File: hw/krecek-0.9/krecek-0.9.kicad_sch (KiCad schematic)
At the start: 0 parts

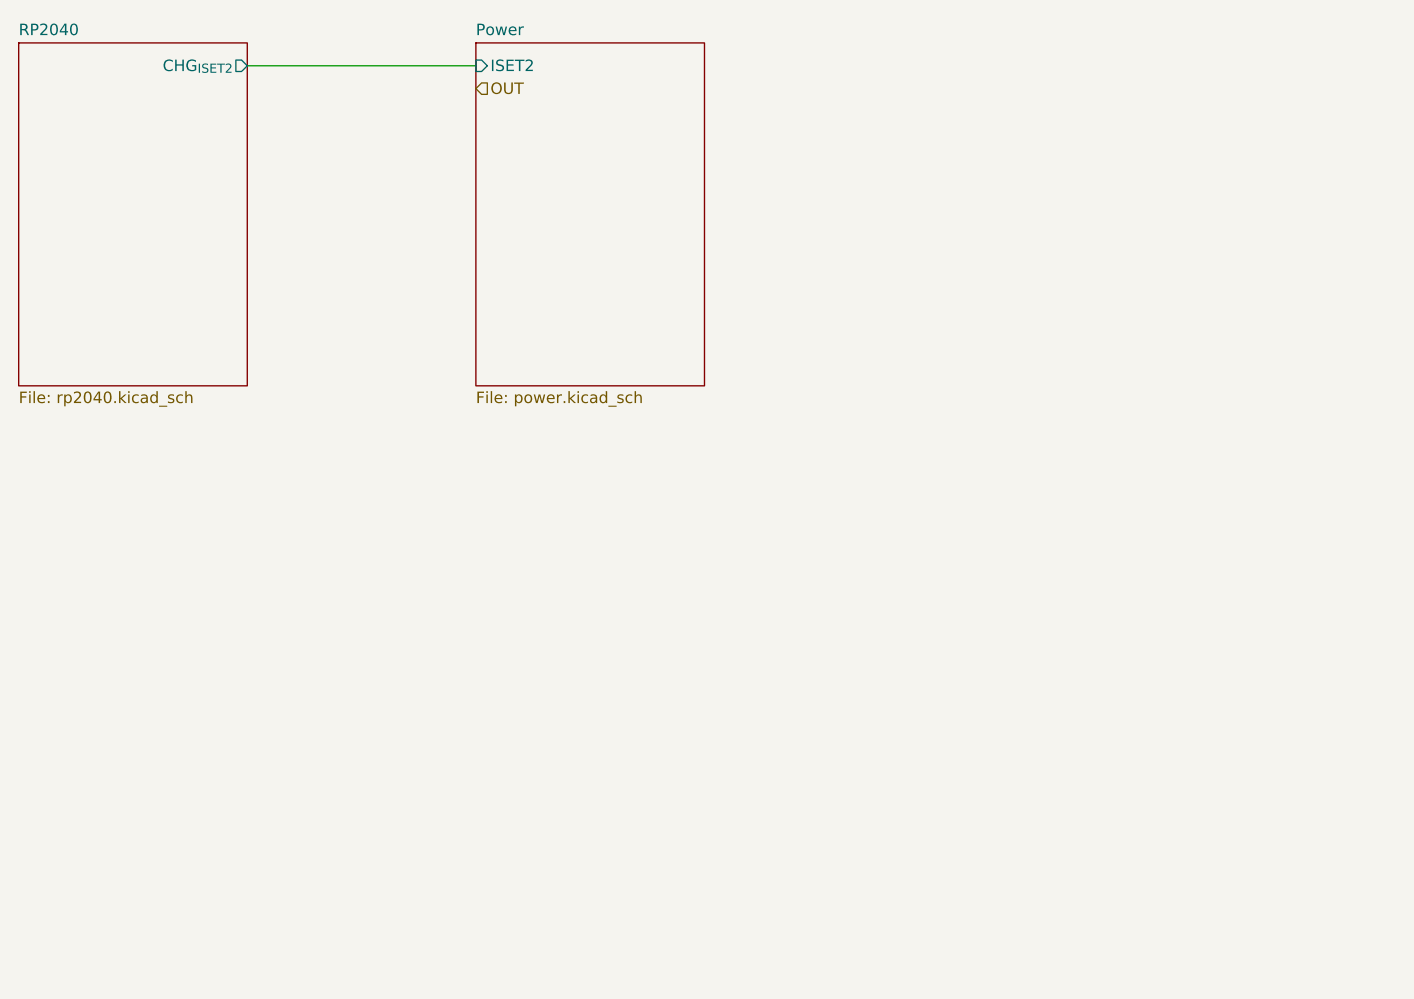
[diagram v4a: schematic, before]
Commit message: Expand hardware design to cover more areas
Signed-off-by: Jan Hamal Dvořák <mordae@anilinux.org>
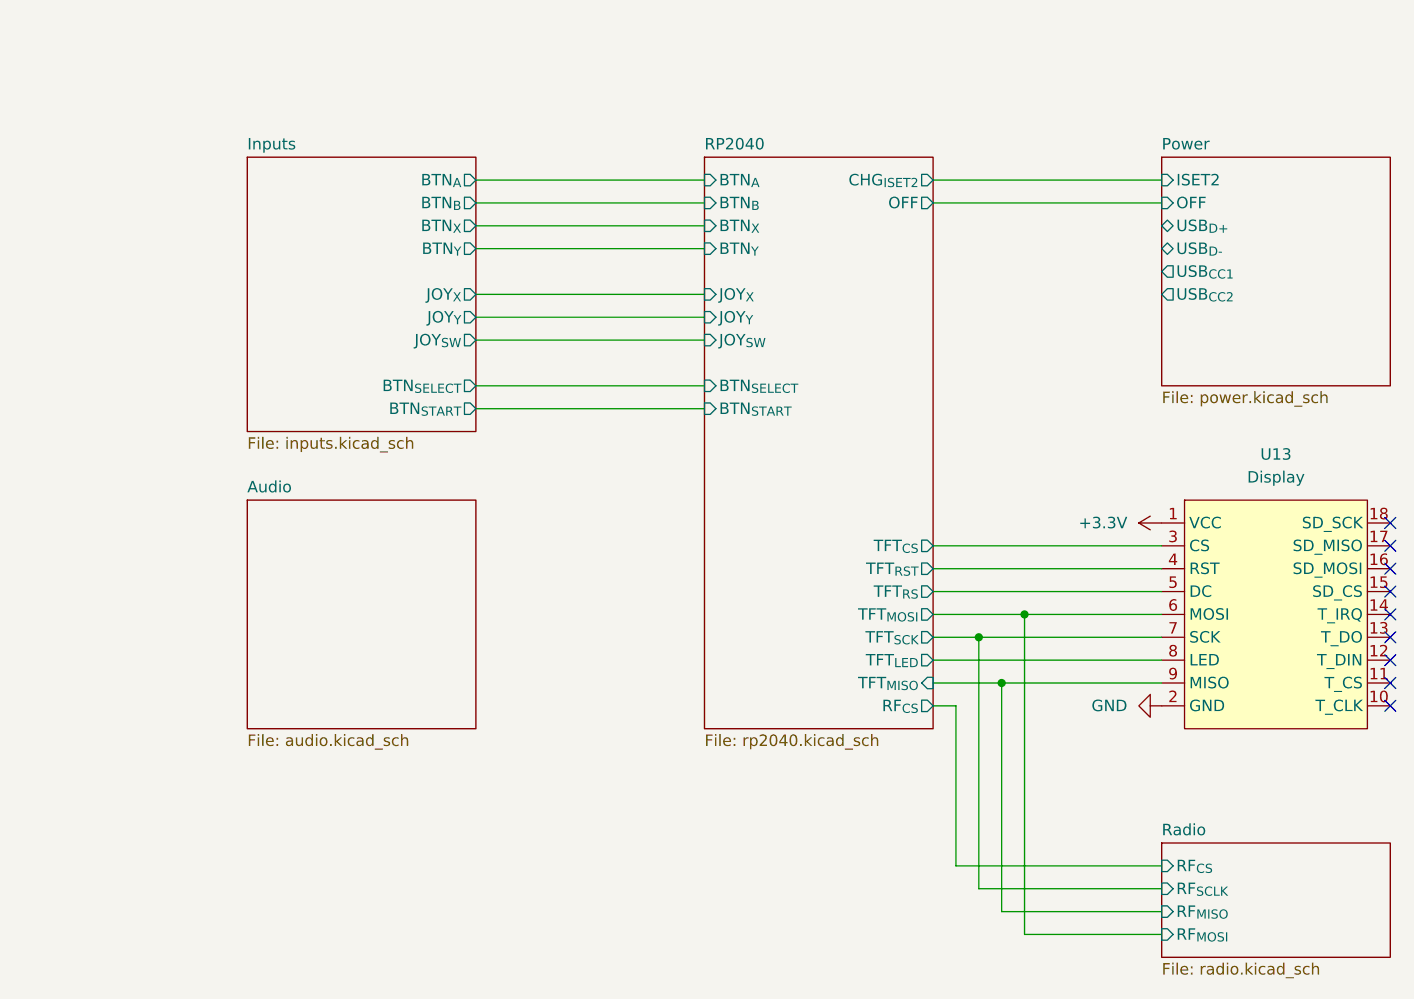
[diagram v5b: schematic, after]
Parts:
- added U13: Display, Krecek:TftDisplay, symbol Krecek:TftDisplay
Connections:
- new net +3.3V: U13.1 (VCC)
- new net GND: U13.2 (GND)
- new net RP2040/TFT_{CS}: U13.3 (CS)
- new net RP2040/TFT_{LED}: U13.8 (LED)
- new net RP2040/TFT_{MISO}: U13.9 (MISO)
- new net RP2040/TFT_{MOSI}: U13.6 (MOSI)
- new net RP2040/TFT_{RST}: U13.4 (RST)
- new net RP2040/TFT_{RS}: U13.5 (DC)
- new net RP2040/TFT_{SCK}: U13.7 (SCK)
- no-connect marks 0 -> 9
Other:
- added sheet Audio (audio.kicad_sch)
- added sheet Inputs (inputs.kicad_sch)
- added sheet Radio (radio.kicad_sch)
- sheet Power ports: added OFF, USB_{CC1}, USB_{CC2}, USB_{D+}, USB_{D-}; removed none
- sheet RP2040 ports: added BTN_{A}, BTN_{B}, BTN_{SELECT}, BTN_{START}, BTN_{X}, BTN_{Y}, JOY_{SW}, JOY_{X}, JOY_{Y}, OFF, RF_{CS}, TFT_{CS}, TFT_{LED}, TFT_{MISO}, TFT_{MOSI}, TFT_{RST}, TFT_{RS}, TFT_{SCK}; removed none
